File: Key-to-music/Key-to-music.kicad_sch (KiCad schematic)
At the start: 3 parts, among them U1 RP2040, U2 W25Q128JVS

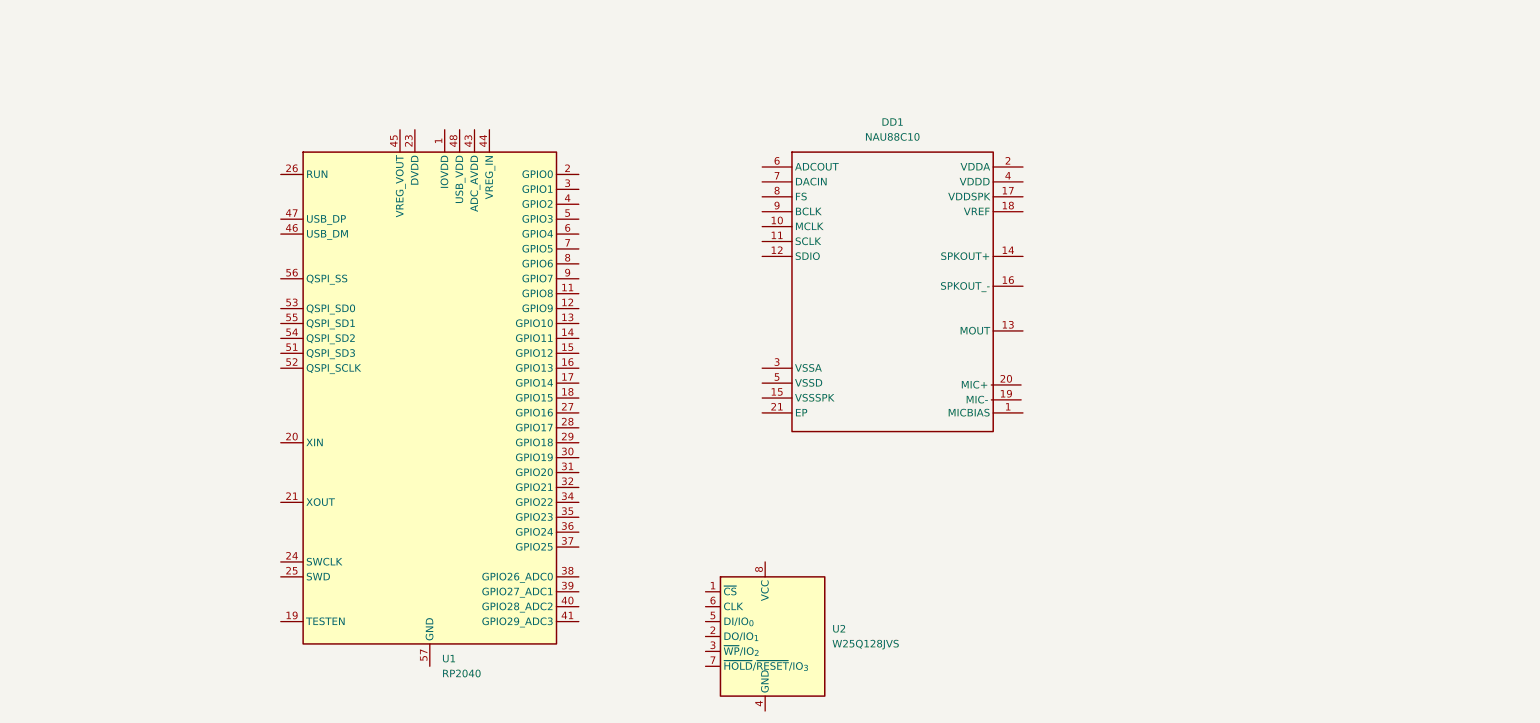
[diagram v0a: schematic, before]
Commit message: Завершена схема и сделана компоновка
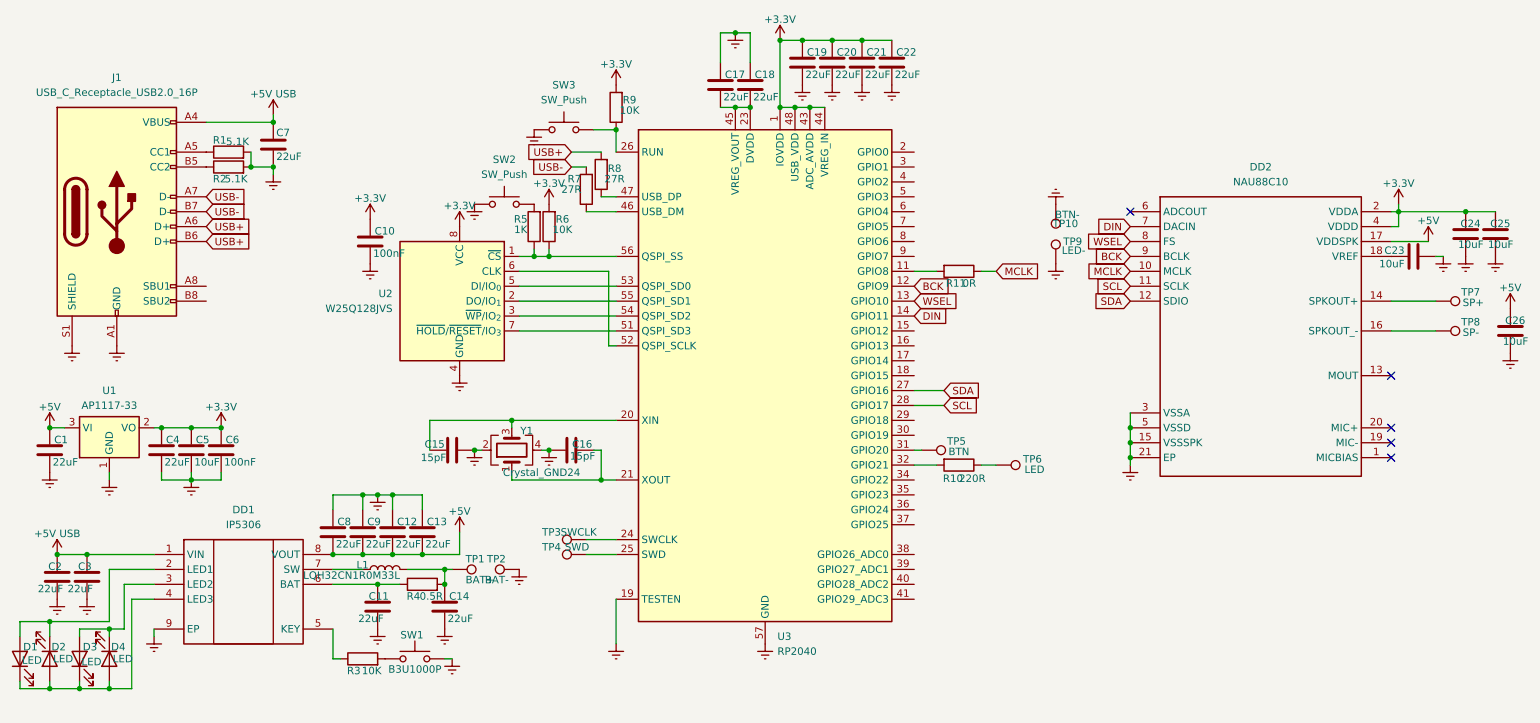
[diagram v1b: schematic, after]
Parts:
- added C1, C11, C12, C13, C14, C17, C18, C19, C2, C20, C21, C22, C3, C4, C7, C8, C9: 22uF, Capacitor_SMD:C_0402_1005Metric, symbol Device:C
- added C10, C6: 100nF, Capacitor_SMD:C_0402_1005Metric, symbol Device:C
- added C15, C16: 15pF, Capacitor_SMD:C_0402_1005Metric, symbol Device:C
- added C23, C24, C25, C26, C5: 10uF, Capacitor_SMD:C_0402_1005Metric, symbol Device:C
- added D1, D2, D3, D4: LED, LED_SMD:LED_0402_1005Metric, symbol Device:LED
- added DD1: IP5306, Package_SO:HSOP-8-1EP_3.9x4.9mm_P1.27mm_EP2.3x2.3mm, symbol IP5306:IP5306
- added J1: USB_C_Receptacle_USB2.0_16P, Connector_USB:USB_C_Receptacle_GCT_USB4105-xx-A_16P_TopMnt_Horizontal, symbol Connector:USB_C_Receptacle_USB2.0_16P
- added L1: LQH32CN1R0M33L, Inductor_SMD:L_1210_3225Metric, symbol Device:L
- added R1, R2: 5.1K, PCM_Resistor_SMD_AKL:R_0402_1005Metric, symbol Device:R
- added R10: 220R, PCM_Resistor_SMD_AKL:R_0402_1005Metric, symbol Device:R
- added R11: 0R, PCM_Resistor_SMD_AKL:R_0402_1005Metric, symbol Device:R
- added R3, R6, R9: 10K, PCM_Resistor_SMD_AKL:R_0402_1005Metric, symbol Device:R
- added R4: 0.5R, PCM_Resistor_SMD_AKL:R_0402_1005Metric, symbol Device:R
- added R5: 1K, PCM_Resistor_SMD_AKL:R_0402_1005Metric, symbol Device:R
- added R7, R8: 27R, PCM_Resistor_SMD_AKL:R_0402_1005Metric, symbol Device:R
- added SW1: B3U1000P, Button_Switch_SMD:SW_SPST_B3U-1000P, symbol Switch:SW_Push
- added SW2, SW3: SW_Push, Button_Switch_SMD:SW_SPST_B3U-1000P, symbol Switch:SW_Push
- added TP1: BAT+, TestPoint:TestPoint_Pad_D2.0mm, symbol Connector:TestPoint
- added TP10: BTN-, TestPoint:TestPoint_Pad_D1.0mm, symbol Connector:TestPoint
- added TP2: BAT-, TestPoint:TestPoint_Pad_D2.0mm, symbol Connector:TestPoint
- added TP3: SWCLK, TestPoint:TestPoint_Pad_D1.0mm, symbol Connector:TestPoint
- added TP4: SWD, TestPoint:TestPoint_Pad_D1.0mm, symbol Connector:TestPoint
- added TP5: BTN, TestPoint:TestPoint_Pad_D1.0mm, symbol Connector:TestPoint
- added TP6: LED, TestPoint:TestPoint_Pad_D1.0mm, symbol Connector:TestPoint
- added TP7: SP+, TestPoint:TestPoint_Pad_D1.0mm, symbol Connector:TestPoint
- added TP8: SP-, TestPoint:TestPoint_Pad_D1.0mm, symbol Connector:TestPoint
- added TP9: LED-, TestPoint:TestPoint_Pad_D1.0mm, symbol Connector:TestPoint
- added U1: AP1117-33, Package_TO_SOT_SMD:SOT-223-3_TabPin2, symbol Regulator_Linear:AP1117-33
- added Y1: Crystal_GND24, Crystal:Crystal_SMD_Abracon_ABM8G-4Pin_3.2x2.5mm, symbol Device:Crystal_GND24
- renumbered DD1 to DD2, U1 to U3
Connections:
- net +3.3V: now reaches U3.1 (IOVDD), U3.10 (IOVDD), U3.22 (IOVDD), U3.33 (IOVDD), U3.42 (IOVDD), U3.49 (IOVDD)
- net +3.3V: now also DD2.2 (VDDA), DD2.4 (VDDD), U2.8 (VCC), U3.43 (ADC_AVDD), U3.44 (VREG_IN), U3.48 (USB_VDD), C10.1, C19.1, C20.1, C21.1, C22.1, C24.2, C25.2, C4.1, C5.1, C6.1, R6.2, R9.2, U1.2 (VO)
- net at U3.11 (GPIO8): now also R11.2
- net BCK: now reaches U3.12 (GPIO9)
- net BCK: now also DD2.9 (BCLK)
- net WSEL: now reaches U3.13 (GPIO10)
- net WSEL: now also DD2.8 (FS)
- net DIN: now reaches U3.14 (GPIO11)
- net DIN: now also DD2.7 (DACIN)
- net Earth: now reaches U3.19 (TESTEN)
- net Earth: now also DD2.15 (VSSSPK), DD2.21 (EP), DD2.3 (VSSA), DD2.5 (VSSD), U2.4 (GND), U3.57 (GND), C1.2, C10.2, C11.2, C12.1, C13.1, C14.2, C15.2, C16.1, C17.1, C18.1, C19.2, C2.2, C20.2, C21.2, C22.2, C23.2, C24.1, C25.1, C26.1, C3.2, C4.2, C5.2, C6.2, C7.2, C8.1, C9.1, DD1.9 (EP), J1.A1 (GND), J1.A12 (GND), J1.B1 (GND), J1.B12 (GND), J1.S1 (SHIELD), R1.2, R2.2, SW1.2, SW2.1, SW3.1, TP10.1, TP2.1, TP9.1, U1.1 (GND), Y1.2, Y1.4
- net at U3.20 (XIN): now also C15.1, Y1.3
- net at U3.21 (XOUT): now also C16.2, Y1.1
- net at U3.23 (DVDD), U3.50 (DVDD): now also U3.45 (VREG_VOUT), C17.2, C18.2
- net at U3.24 (SWCLK): now also TP3.1
- net at U3.25 (SWD): now also TP4.1
- net at U3.26 (RUN): now also R9.1, SW3.2
- net SDA: now reaches U3.27 (GPIO16)
- net SDA: now also DD2.12 (SDIO)
- net SCL: now reaches U3.28 (GPIO17)
- net SCL: now also DD2.11 (SCLK)
- net at U3.31 (GPIO20): now also TP5.1
- net at U3.32 (GPIO21): now also R10.2
- net at U3.46 (USB_DM): now also R7.1
- net at U3.47 (USB_DP): now also R8.1
- net at U3.51 (QSPI_SD3): now also U2.7 (~{HOLD}/~{RESET}/IO_{3})
- net at U3.52 (QSPI_SCLK): now also U2.6 (CLK)
- net at U3.53 (QSPI_SD0): now also U2.5 (DI/IO_{0})
- net at U3.54 (QSPI_SD2): now also U2.3 (~{WP}/IO_{2})
- net at U3.55 (QSPI_SD1): now also U2.2 (DO/IO_{1})
- net at U3.56 (QSPI_SS): now also U2.1 (~{CS}), R5.1, R6.1
- net MCLK: now reaches DD2.10 (MCLK)
- net MCLK: now also R11.1
- net at DD2.14 (SPKOUT+): now also TP7.1
- net at DD2.16 (SPKOUT_-): now also TP8.1
- net +5V: now reaches DD2.17 (VDDSPK)
- net +5V: now also C1.1, C12.2, C13.2, C26.2, C8.2, C9.2, DD1.8 (VOUT), U1.3 (VI)
- net at DD2.18 (VREF): now also C23.1
- new net: R3.2, SW1.1
- new net: J1.B5 (CC2), R2.1
- new net: R5.2, SW2.2
- new net: DD1.7 (SW), L1.1
- new net: C14.1, L1.2, R4.2, TP1.1
- new net: C11.1, DD1.6 (BAT), R4.1
- new net: D1.2 (A), D2.1 (K), DD1.2 (LED1)
- new net: D3.2 (A), D4.1 (K), DD1.3 (LED2)
- new net: D1.1 (K), D2.2 (A), D3.1 (K), D4.2 (A), DD1.4 (LED3)
- new net: DD1.5 (KEY), R3.1
- new net: J1.A5 (CC1), R1.1
- new net: R10.1, TP6.1
- new net +5V USB: C2.1, C3.1, C7.1, DD1.1 (VIN), J1.A4 (VBUS), J1.A9 (VBUS), J1.B4 (VBUS), J1.B9 (VBUS)
- new net USB+: J1.A6 (D+), J1.B6 (D+), R8.2
- new net USB-: J1.A7 (D-), J1.B7 (D-), R7.2
- no-connect marks 0 -> 5
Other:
- moved on the sheet: DD2, U2, U3

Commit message: rev0 готова
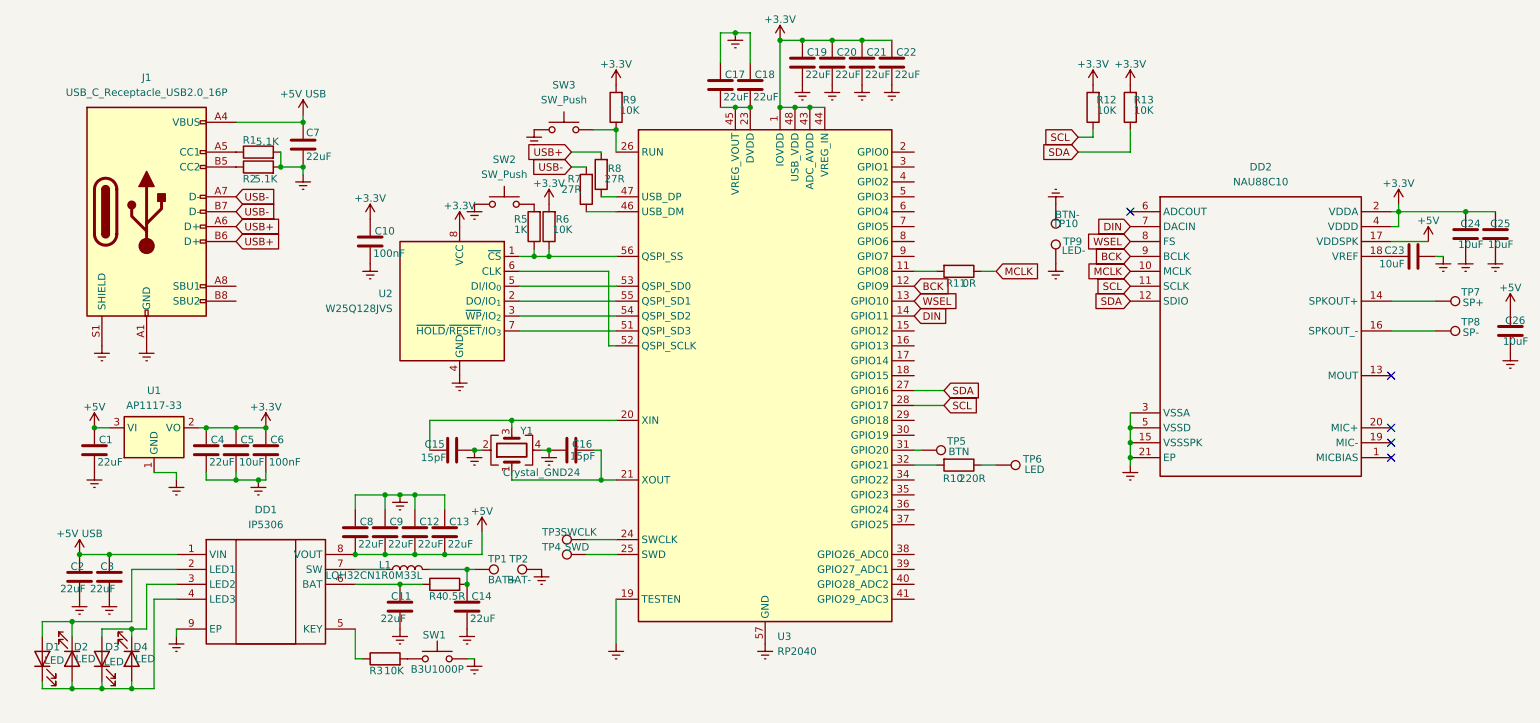
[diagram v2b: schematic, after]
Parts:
- added R12, R13: 10K, PCM_Resistor_SMD_AKL:R_0402_1005Metric, symbol Device:R
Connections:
- net +3.3V: now also R12.2, R13.2
- net SCL: now also R12.1
- net SDA: now also R13.1
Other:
- moved on the sheet: C1, C11, C12, C13, C14, C2, C3, C4, C5, C6, C7, C8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
